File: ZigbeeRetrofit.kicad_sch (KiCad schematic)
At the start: 24 parts, among them J1 110990030, J2 U.FL-R-SMT-1(10), J3 TC2050-IDC-NL, U1 CC2531F256RHAT, U2 SPX3819M5-L-3-3, Y1 32 Mhz, Y2 ECS-.327-12.5-34RR-TR

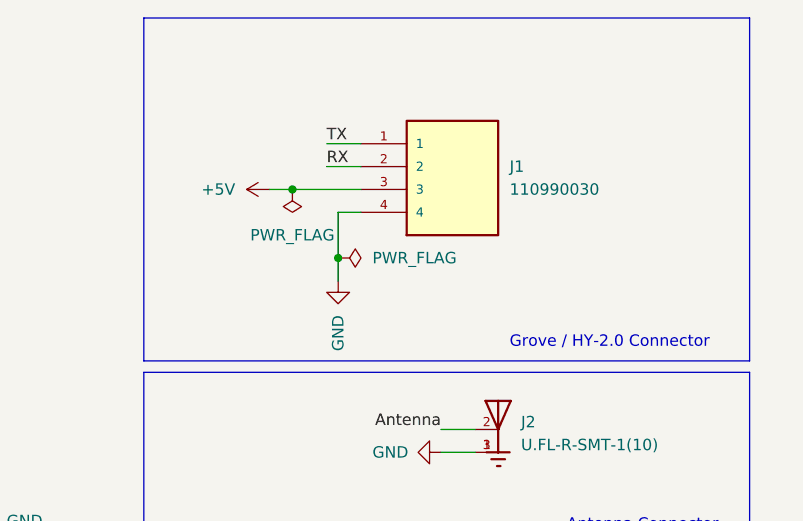
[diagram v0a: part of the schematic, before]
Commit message: Updated grove connector
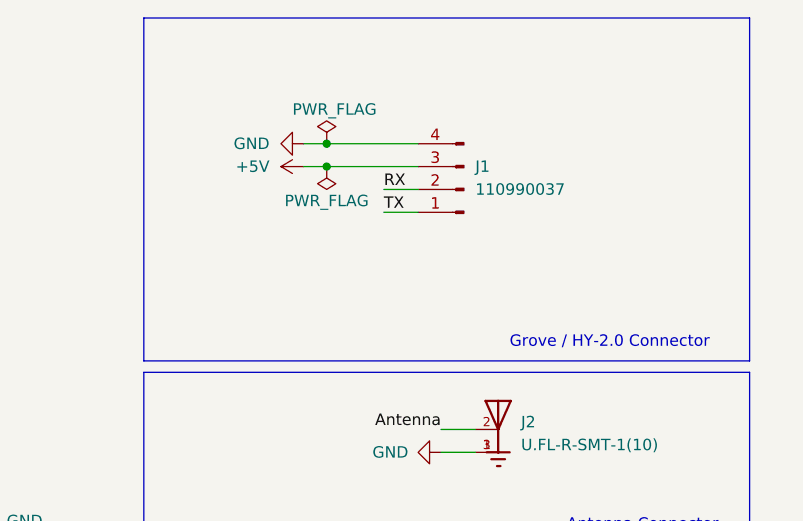
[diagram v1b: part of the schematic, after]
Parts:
- J1: value 110990030 -> 110990037; footprint 110990030:SEEED_110990030 -> Connector_JST:JST_PH_S4B-PH-K_1x04_P2.00mm_Horizontal; symbol 110990030:110990030 -> Connector:Conn_01x04_Male; Check_prices https://www.snapeda.com/parts/114020164/Seeed+Technology+Co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 -> (none); MP 114020164 -> 110990037; Purchase-URL https://www.snapeda.com/api/url_track_click_mouser/?unipart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 -> (none); SnapEDA_Link https://www.snapeda.com/parts/114020164/Seeed+Technology+Co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 -> (none)
